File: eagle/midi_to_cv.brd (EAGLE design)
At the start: 100 x 80 mm, 66 parts, among them IC1 4093N, Q3 2N3904, Q4 2N3904, Q5 2N3904, Q6 2SK30, U1 ATMEGA328P_PDIP

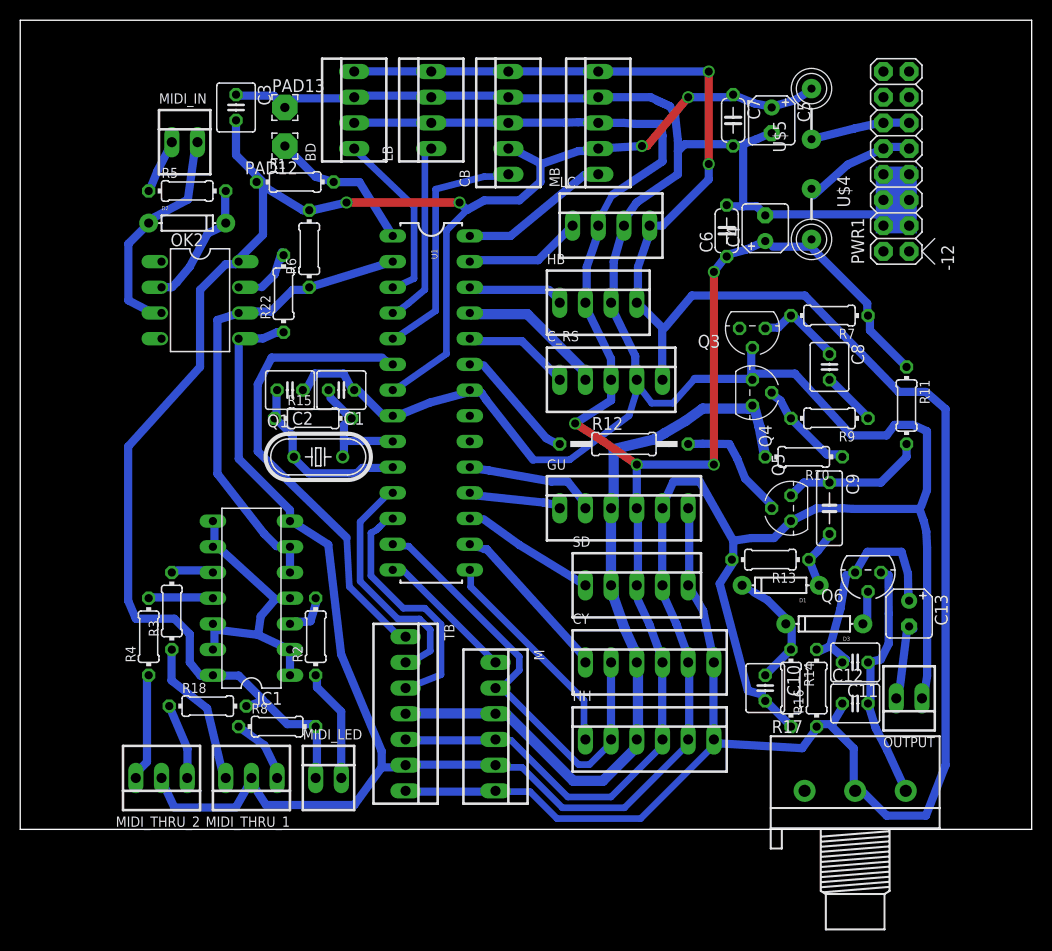
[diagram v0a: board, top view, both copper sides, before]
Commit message: tweaks
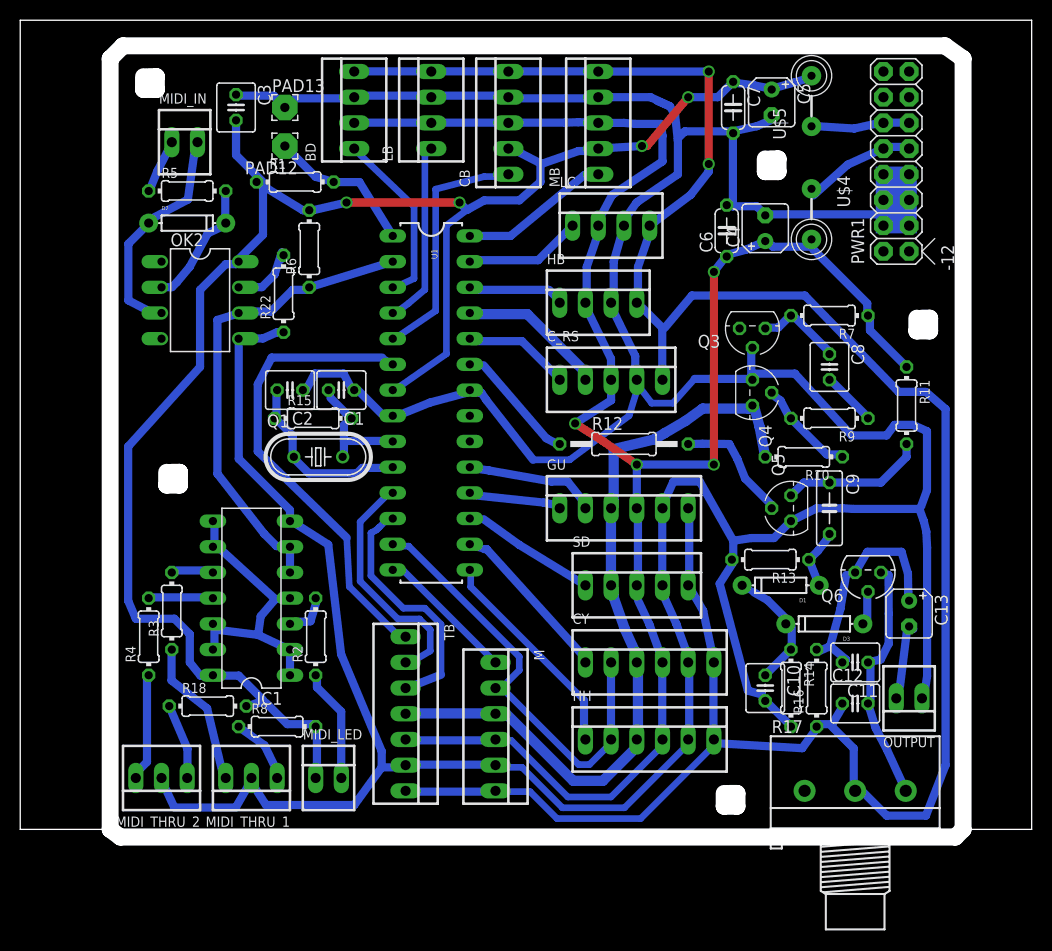
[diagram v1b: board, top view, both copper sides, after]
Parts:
- moved C5 1.78 mm to (74.3, 71.9)
- moved C7 1.27 mm to (70.5, 71.4)
- moved U$5 1.27 mm to (78.2, 72.0)
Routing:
- net GND: track 424.6 -> 426.9 mm
- net RETURN: track 235.3 -> 234.8 mm
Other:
- board size 100 x 80 mm -> 100 x 80.8 mm
